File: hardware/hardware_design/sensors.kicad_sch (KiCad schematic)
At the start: 17 parts, among them Q1 TEMT6000X01, U2 MAX4466EXK, U7 BME280

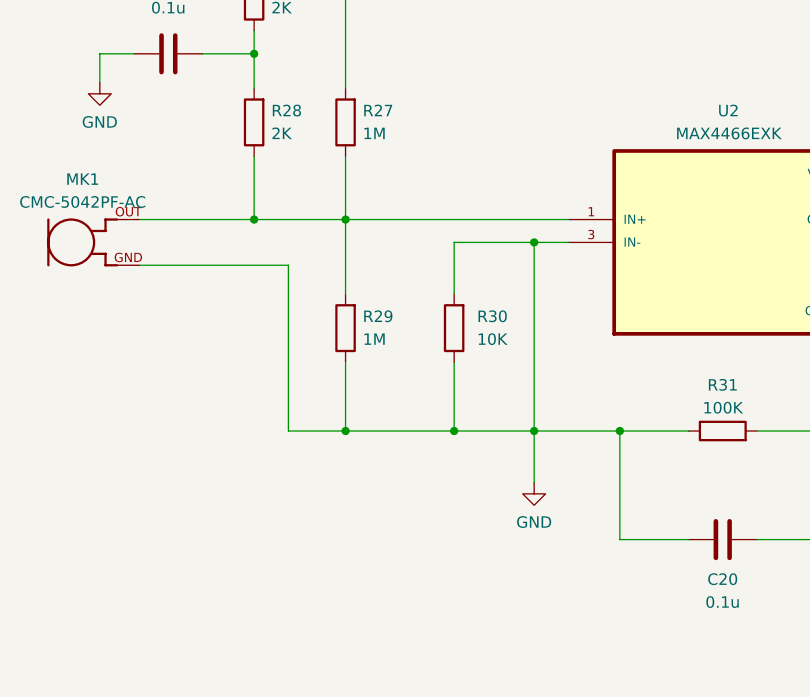
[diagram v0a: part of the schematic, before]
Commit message: pcb layout completed
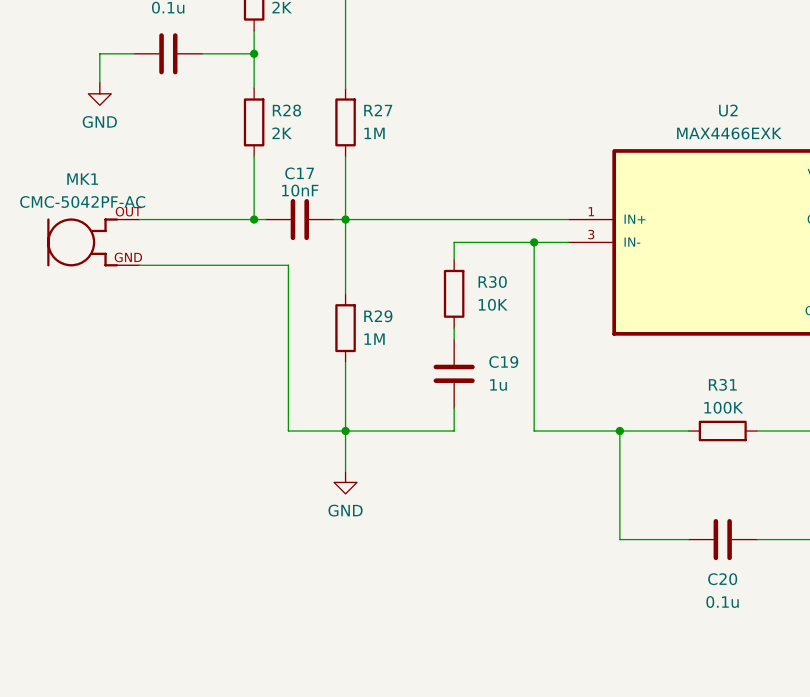
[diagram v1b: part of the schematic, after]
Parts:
- added C17: 10nF, Capacitor_SMD:C_0805_2012Metric, symbol Device:C
- added C19: 1u, Capacitor_SMD:C_0805_2012Metric, symbol Device:C
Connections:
- net GND: now also C19.2; no longer C20.1, R30.1, R30.2, R31.1, U2.3 (IN-)
- net at R27.1, R29.2, U2.1 (IN+): now also C17.2; no longer MK1.OUT, R28.1
- new net: C19.1, R30.1
- new net: C20.1, R30.2, R31.1, U2.3 (IN-)
- new net: C17.1, MK1.OUT, R28.1
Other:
- moved on the sheet: R30
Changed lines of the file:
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@@
-	)
-	(junction
-		(at 78.74 160.02)
-		(diameter 0)
-		(color 0 0 0 0)
 	)
 	(junction
@@
 	)
 	(junction
-		(at 69.85 160.02)
-		(diameter 0)
-		(color 0 0 0 0)
-	)
-	(junction
 		(at 238.76 92.71)
 		(diameter 0)
@@
 	(wire
 		(pts
-			(xy 78.74 160.02) (xy 78.74 165.735)
-		)
-		(stroke
-			(width 0)
-			(type default)
-		)
-	)
-	(wire
-		(pts
 			(xy 238.76 92.71) (xy 238.76 97.79)
 		)
@@
 	(wire
 		(pts
-			(xy 69.85 160.02) (xy 78.74 160.02)
-		)
-		(stroke
-			(width 0)
-			(type default)
-		)
-	)
-	(wire
-		(pts
 			(xy 238.76 72.39) (xy 238.76 74.93)
 		)
@@
 	(wire
 		(pts
-			(xy 69.85 152.4) (xy 69.85 160.02)
+			(xy 69.85 148.59) (xy 69.85 149.86)
 		)
 		(stroke
@@
 	(wire
 		(pts
+			(xy 69.85 157.48) (xy 69.85 160.02)
+		)
+		(stroke
+			(width 0)
+			(type default)
+		)
+	)
+	(wire
+		(pts
+			(xy 56.515 136.525) (xy 57.785 136.525)
+		)
+		(stroke
+			(width 0)
+			(type default)
+		)
+	)
+	(wire
+		(pts
 			(xy 232.41 74.93) (xy 238.76 74.93)
 		)
@@
 	(wire
 		(pts
+			(xy 57.785 160.02) (xy 57.785 164.465)
+		)
+		(stroke
+			(width 0)
+			(type default)
+		)
+	)
+	(wire
+		(pts
 			(xy 175.26 71.12) (xy 175.26 62.23)
 		)
@@
 	(wire
 		(pts
-			(xy 69.85 144.78) (xy 69.85 139.065)
+			(xy 69.85 140.97) (xy 69.85 139.065)
 		)
 		(stroke
@@
 	(wire
 		(pts
-			(xy 47.625 136.525) (xy 57.785 136.525)
+			(xy 47.625 136.525) (xy 48.895 136.525)
 		)
 		(stroke
@@
 	(symbol
 		(lib_id "Device:R")
-		(at 69.85 148.59 180)
+		(at 69.85 144.78 180)
 		(unit 1)
 		(body_style 1)
@@
 		(fields_autoplaced yes)
 		(property "Reference" "R30"
-			(at 72.39 147.3199 0)
+			(at 72.39 143.5099 0)
 			(show_name no)
 			(do_not_autoplace no)
@@
 		)
 		(property "Value" "10K"
-			(at 72.39 149.8599 0)
+			(at 72.39 146.0499 0)
 			(show_name no)
 			(do_not_autoplace no)
@@
 		)
 		(property "Footprint" "Resistor_SMD:R_0805_2012Metric"
-			(at 71.628 148.59 90)
+			(at 71.628 144.78 90)
 			(hide yes)
 			(show_name no)
@@
 		)
 		(property "Datasheet" ""
-			(at 69.85 148.59 0)
+			(at 69.85 144.78 0)
 			(hide yes)
 			(show_name no)
@@
 		)
 		(property "Description" "Resistor"
-			(at 69.85 148.59 0)
+			(at 69.85 144.78 0)
 			(hide yes)
 			(show_name no)
@@
 	)
 	(symbol
+		(lib_id "Device:C")
+		(at 52.705 136.525 90)
+		(unit 1)
+		(body_style 1)
+		(exclude_from_sim no)
+		(in_bom yes)
+		(on_board yes)
+		(in_pos_files yes)
+		(dnp no)
+		(property "Reference" "C17"
+			(at 52.705 131.445 90)
+			(show_name no)
+			(do_not_autoplace no)
+			(effects
+				(font
+					(size 1.27 1.27)
+				)
+			)
+		)
+		(property "Value" "10nF"
+			(at 52.705 133.35 90)
+			(show_name no)
+			(do_not_autoplace no)
+			(effects
+				(font
+					(size 1.27 1.27)
+				)
+			)
+		)
+		(property "Footprint" "Capacitor_SMD:C_0805_2012Metric"
+			(at 56.515 135.5598 0)
+			(hide yes)
+			(show_name no)
+			(do_not_autoplace no)
+			(effects
+				(font
+					(size 1.27 1.27)
+				)
+			)
+		)
+		(property "Datasheet" ""
+			(at 52.705 136.525 0)
+			(hide yes)
+			(show_name no)
+			(do_not_autoplace no)
+			(effects
+				(font
+					(size 1.27 1.27)
+				)
+			)
+		)
+		(property "Description" "Unpolarized capacitor"
+			(at 52.705 136.525 0)
+			(hide yes)
+			(show_name no)
+			(do_not_autoplace no)
+			(effects
+				(font
+					(size 1.27 1.27)
+				)
+			)
+		)
+		(pin "1"
+		)
+		(pin "2"
+		)
+		(instances
+			(project "ESP32 IoT 4-layer PCB"
+				(path "/e6224326-a3f2-4f93-9736-980cb0b8e09e/379ef173-1d07-4055-8876-f4e521633af1/e1d26e0e-f6e0-4a69-be04-9682b536d32e"
+					(reference "C17")
+					(unit 1)
+				)
+			)
+		)
+	)
+	(symbol
 		(lib_id "Device:R")
 		(at 185.42 74.93 0)
@@
 	(symbol
 		(lib_id "power:GND")
-		(at 78.74 165.735 0)
+		(at 57.785 164.465 0)
 		(unit 1)
 		(body_style 1)
@@
 		(fields_autoplaced yes)
 		(property "Reference" "#PWR041"
-			(at 78.74 172.085 0)
+			(at 57.785 170.815 0)
 			(hide yes)
 			(show_name no)
@@
 		)
 		(property "Value" "GND"
-			(at 78.74 170.18 0)
+			(at 57.785 168.91 0)
 			(show_name no)
 			(do_not_autoplace no)
@@
 		)
 		(property "Footprint" ""
-			(at 78.74 165.735 0)
+			(at 57.785 164.465 0)
 			(hide yes)
 			(show_name no)
@@
 		)
 		(property "Datasheet" ""
-			(at 78.74 165.735 0)
+			(at 57.785 164.465 0)
 			(hide yes)
 			(show_name no)
@@
 		)
 		(property "Description" "Power symbol creates a global label with name \"GND\" , ground"
-			(at 78.74 165.735 0)
+			(at 57.785 164.465 0)
 			(hide yes)
 			(show_name no)
@@
 					(unit 1)
 				)
+			)
+		)
+	)
+	(symbol
+		(lib_id "Device:C")
+		(at 69.85 153.67 0)
+		(unit 1)
+		(body_style 1)
+		(exclude_from_sim no)
+		(in_bom yes)
+		(on_board yes)
+		(in_pos_files yes)
+		(dnp no)
+		(fields_autoplaced yes)
+		(property "Reference" "C19"
+			(at 73.66 152.3999 0)
+			(show_name no)
+			(do_not_autoplace no)
+			(effects
+				(font
+					(size 1.27 1.27)
+				)
+				(justify left)
+			)
+		)
+		(property "Value" "1u"
+			(at 73.66 154.9399 0)
+			(show_name no)
+			(do_not_autoplace no)
+			(effects
+				(font
+					(size 1.27 1.27)
+				)
+				(justify left)
+			)
+		)
+		(property "Footprint" "Capacitor_SMD:C_0805_2012Metric"
+			(at 70.8152 157.48 0)
+			(hide yes)
+			(show_name no)
+			(do_not_autoplace no)
+			(effects
+				(font
+					(size 1.27 1.27)
+				)
+			)
+		)
+		(property "Datasheet" ""
+			(at 69.85 153.67 0)
+			(hide yes)
+			(show_name no)
+			(do_not_autoplace no)
+			(effects
+				(font
+					(size 1.27 1.27)
+				)
+			)
+		)
+		(property "Description" "Unpolarized capacitor"
+			(at 69.85 153.67 0)
+			(hide yes)
+			(show_name no)
+			(do_not_autoplace no)
+			(effects
+				(font
+					(size 1.27 1.27)
+				)
+			)
+		)
+		(pin "1"
+		)
+		(pin "2"
+		)
+		(instances
+			(project "ESP32 IoT 4-layer PCB"
+				(path "/e6224326-a3f2-4f93-9736-980cb0b8e09e/379ef173-1d07-4055-8876-f4e521633af1/e1d26e0e-f6e0-4a69-be04-9682b536d32e"
+					(reference "C19")
+					(unit 1)
+				)
